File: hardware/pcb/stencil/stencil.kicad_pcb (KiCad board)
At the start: 2 copper layers, 19 x 48.2 mm, 25 parts, among them J1 USB_A, J2 Conn_01x10, J2 FH34SRJ-12S-0.5SH, J3 FH34SRJ-12S-0.5SH, J4 Conn_01x05, U2 AP2112K-3.3, U3 NC7SB3157P6X, U4 NC7SB3157P6X, U5 PRTR5V0U2X

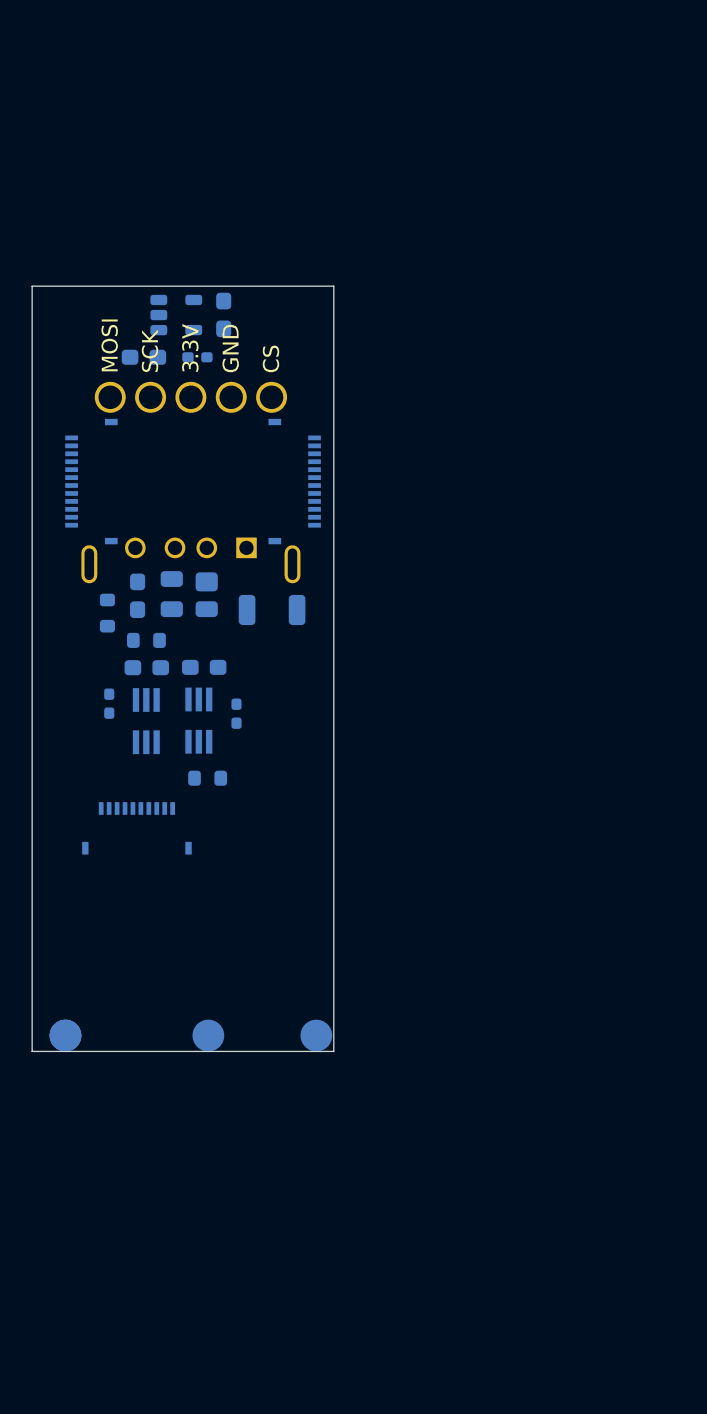
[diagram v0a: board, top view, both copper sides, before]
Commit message: production
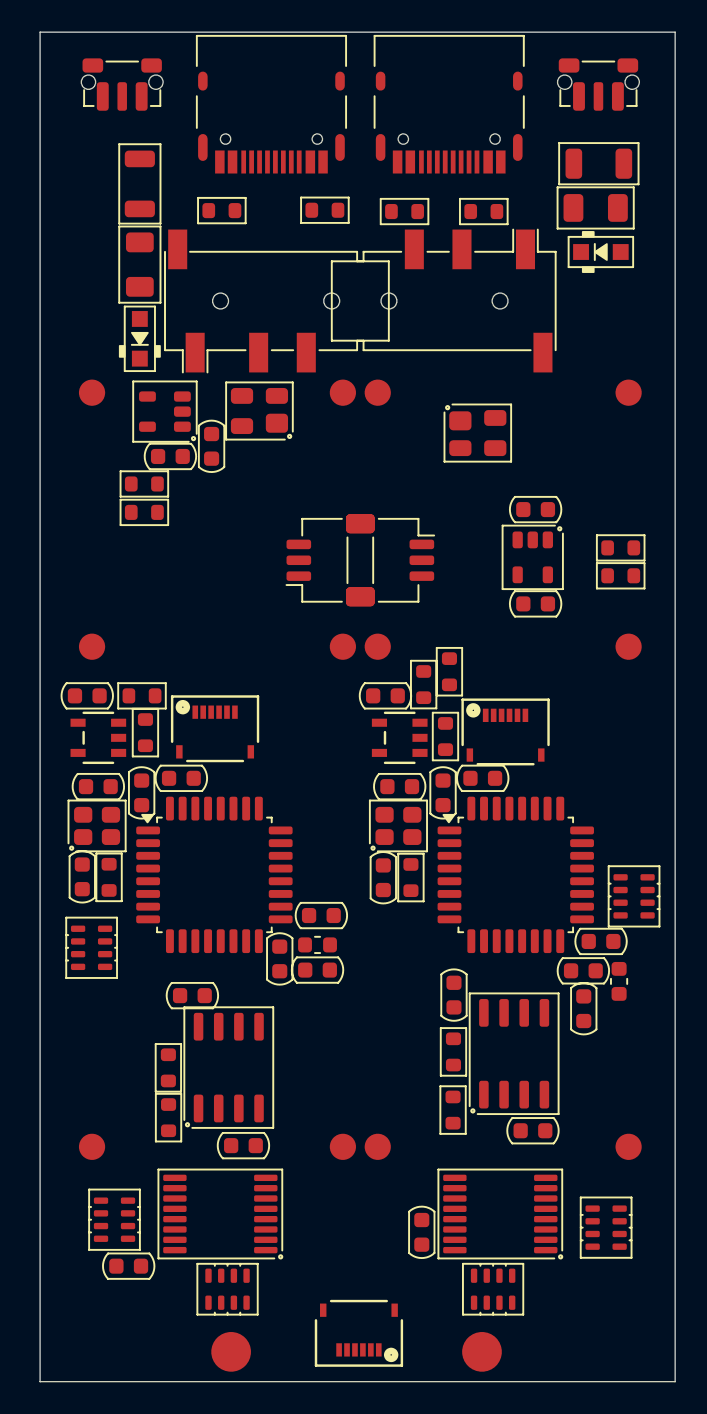
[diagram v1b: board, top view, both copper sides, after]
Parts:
- removed C1: C_Small, PCM_Capacitor_SMD_AKL:C_0603_1608Metric_Pad1.05x0.95mm
- removed the C2 at (112.1, 117.8)
- removed the C3 at (107.0, 120.5)
- removed the C6 at (110.8, 140.0)
- removed the C7 at (107.2, 140.0)
- removed the J1 at (110.0, 133.0)
- removed the J2 at (106.6, 150.1)
- removed the J2 at (103.7, 128.3)
- removed the J3 at (116.5, 128.3)
- removed the J4 at (110.0, 123.0)
- removed the L1 at (115.1, 136.4)
- removed the R1 at (110.4, 120.5)
- removed the R2 at (104.9, 142.3)
- removed the R3 at (112.9, 142.9)
- removed the R6 at (107.2, 138.3)
- removed the R7 at (111.1, 147.0)
- removed REF** (x4): NPTH, NPTH
- removed the U2 at (109.1, 117.8)
- removed the U3 at (110.5, 143.4)
- removed the U4 at (107.2, 143.4)
- removed the U5 at (109.9, 135.4)
- added C10: 220pF, PCM_Capacitor_SMD_AKL:C_0603_1608Metric, F.Cu at (131.5, 169.2)
- added C10: 220pF, PCM_Capacitor_SMD_AKL:C_0603_1608Metric, F.Cu at (113.3, 170.1)
- added C11: 4.7 uF, PCM_Capacitor_SMD_AKL:C_0603_1608Metric, F.Cu at (135.8, 157.3)
- added C12: 1u, PCM_Capacitor_SMD_AKL:C_0603_1608Metric, F.Cu at (134.7, 159.1)
- added C13: 10n, PCM_Capacitor_SMD_AKL:C_0603_1608Metric, F.Cu at (134.7, 161.5)
- added C14: 10n, PCM_Capacitor_SMD_AKL:C_0603_1608Metric, F.Cu at (103.5, 141.8)
- added C14: 10n, PCM_Capacitor_SMD_AKL:C_0603_1608Metric, F.Cu at (122.3, 141.8)
- added C15: 4.7 uF, PCM_Capacitor_SMD_AKL:C_0603_1608Metric, F.Cu at (109.4, 147.0)
- added C16: 10n, PCM_Capacitor_SMD_AKL:C_0603_1608Metric, F.Cu at (118.0, 159.1)
- added C17: 1u, PCM_Capacitor_SMD_AKL:C_0603_1608Metric, F.Cu at (115.6, 158.4)
- added C2: 0.1uF, PCM_Capacitor_SMD_AKL:C_0603_1608Metric, F.Cu at (110.1, 160.7)
- added C2: 0.1uF, PCM_Capacitor_SMD_AKL:C_0603_1608Metric, F.Cu at (126.6, 160.7)
- added C3: 0.1uF, PCM_Capacitor_SMD_AKL:C_0603_1608Metric, F.Cu at (106.1, 177.7)
- added C3: 0.1uF, PCM_Capacitor_SMD_AKL:C_0603_1608Metric, F.Cu at (124.5, 175.6)
- added C4: 0.1uF, PCM_Capacitor_SMD_AKL:C_0603_1608Metric, F.Cu at (118.2, 155.6)
- added C4: 0.1uF, PCM_Capacitor_SMD_AKL:C_0603_1608Metric, F.Cu at (128.4, 147.0)
- added C5: 0.1uF, PCM_Capacitor_SMD_AKL:C_0603_1608Metric, F.Cu at (106.9, 147.9)
- added C5: 0.1uF, PCM_Capacitor_SMD_AKL:C_0603_1608Metric, F.Cu at (125.9, 147.9)
- added C6: 10pF, PCM_Capacitor_SMD_AKL:C_0603_1608Metric, F.Cu at (104.2, 147.5)
- added C6: 10pF, PCM_Capacitor_SMD_AKL:C_0603_1608Metric, F.Cu at (123.2, 147.5)
- added C7: 10pF, PCM_Capacitor_SMD_AKL:C_0603_1608Metric, F.Cu at (103.2, 153.2)
- added C7: 10pF, PCM_Capacitor_SMD_AKL:C_0603_1608Metric, F.Cu at (122.1, 153.3)
- added C8: 1uF, PCM_Capacitor_SMD_AKL:C_0603_1608Metric, F.Cu at (108.7, 126.7)
- added C8: 1uF, PCM_Capacitor_SMD_AKL:C_0603_1608Metric, F.Cu at (131.7, 130.1)
- added C9: 1uF, PCM_Capacitor_SMD_AKL:C_0603_1608Metric, F.Cu at (111.3, 126.1)
- added C9: 1uF, PCM_Capacitor_SMD_AKL:C_0603_1608Metric, F.Cu at (131.7, 136.0)
- added D1: 1N5819, PCM_Diode_SMD_AKL:D_SOD-323_HandSoldering, F.Cu at (135.8, 113.8)
- added D1: 1N5819, PCM_Diode_SMD_AKL:D_SOD-323_HandSoldering, F.Cu at (106.8, 119.3)
- added F1: 500mA, PCM_Fuse_AKL:Fuse_1206_3216Metric, F.Cu at (106.8, 114.6)
- added F1: 500mA, PCM_Fuse_AKL:Fuse_1206_3216Metric, F.Cu at (135.5, 111.1)
- added FB1: 1kΩ 100mhz, Inductor_SMD:L_0603_1608Metric, F.Cu at (137.0, 159.8)
- added FB1: 1kΩ 100mhz, Inductor_SMD:L_0603_1608Metric, F.Cu at (118.0, 157.5)
- added H13: ~, ec_parts:SMT-SO-M1.6-screwhole_only, F.Cu at (103.8, 170.2)
- added H13: ~, ec_parts:SMT-SO-M1.6-screwhole_only, F.Cu at (137.6, 170.2)
- added H14: ~, ec_parts:SMT-SO-M1.6-screwhole_only, F.Cu at (137.6, 122.7)
- added H14: ~, ec_parts:SMT-SO-M1.6-screwhole_only, F.Cu at (103.8, 122.7)
- added H15: ~, ec_parts:SMT-SO-M1.6-screwhole_only, F.Cu at (121.8, 122.7)
- added H15: ~, ec_parts:SMT-SO-M1.6-screwhole_only, F.Cu at (119.6, 122.7)
- added H16: ~, ec_parts:SMT-SO-M1.6-screwhole_only, F.Cu at (119.6, 170.2)
- added H16: ~, ec_parts:SMT-SO-M1.6-screwhole_only, F.Cu at (121.8, 170.2)
- added H18: ~, ec_parts:SMT-SO-M1.6-screwhole_only, F.Cu at (103.8, 138.7)
- added H18: ~, ec_parts:SMT-SO-M1.6-screwhole_only, F.Cu at (121.8, 138.7)
- added H19: ~, ec_parts:SMT-SO-M1.6-screwhole_only, F.Cu at (119.6, 138.7)
- added H19: ~, ec_parts:SMT-SO-M1.6-screwhole_only, F.Cu at (137.6, 138.7)
- added H3: ~, ec_parts:SMT-SO-M1.6-with-ring, F.Cu at (128.3, 183.1)
- added H4: ~, ec_parts:SMT-SO-M1.6-with-ring, F.Cu at (112.5, 183.1)
- added J1: SM03B-SRSS-TB, Connector_JST:JST_SH_SM03B-SRSS-TB_1x03-1MP_P1.00mm_Horizontal, F.Cu at (118.8, 133.3)
- added J1: SM04B-SRSS-TB, Connector_JST:JST_SH_SM03B-SRSS-TB_1x03-1MP_P1.00mm_Horizontal, F.Cu at (122.5, 133.3)
- added J2: PJ320D, ec_parts:Jack_3.5mm_PJ320D_Horizontal, F.Cu at (114.1, 116.9)
- added J2: PJ320D, ec_parts:Jack_3.5mm_PJ320D_Horizontal, F.Cu at (127.2, 116.9)
- added J3: HRO_TYPE-C-31-M-12, ec_parts:USB_C_Receptacle_HRO_TYPE-C-31-M-12, F.Cu at (126.3, 104.1)
- added J3: HRO_TYPE-C-31-M-12, ec_parts:USB_C_Receptacle_HRO_TYPE-C-31-M-12, F.Cu at (115.1, 104.1)
- added J4: HRS_FH34SRJ-06S-0.5SH(50), ec_parts:CONN6x1_FH34SRJ-6S-0.5SH50_HIR, F.Cu at (129.8, 144.1)
- added J4: HRS_FH34SRJ-06S-0.5SH(50), ec_parts:CONN6x1_FH34SRJ-6S-0.5SH50_HIR, F.Cu at (120.6, 182.0)
- added J4: HRS_FH34SRJ-06S-0.5SH(50), ec_parts:CONN6x1_FH34SRJ-6S-0.5SH50_HIR, F.Cu at (111.5, 143.9)
- added L1: 60R@100MHz, PCM_Inductor_SMD_AKL:L_1206_3216Metric, F.Cu at (106.8, 109.6)
- added L1: 60R@100MHz, PCM_Inductor_SMD_AKL:L_1206_3216Metric, F.Cu at (135.7, 108.3)
- added R1: 10k, PCM_Resistor_SMD_AKL:R_0603_1608Metric, F.Cu at (123.9, 153.2)
- added R1: 10k, PCM_Resistor_SMD_AKL:R_0603_1608Metric, F.Cu at (107.1, 128.5)
- added R10: 10k, PCM_Resistor_SMD_AKL:R_0603_1608Metric, F.Cu at (126.0, 144.4)
- added R10: 10k, PCM_Resistor_SMD_AKL:R_0603_1608Metric, F.Cu at (107.1, 144.1)
- added R2: 5.1k, PCM_Resistor_SMD_AKL:R_0603_1608Metric, F.Cu at (118.4, 111.2)
- added R2: 5.1k, PCM_Resistor_SMD_AKL:R_0603_1608Metric, F.Cu at (128.4, 111.3)
- added R3: 5.1k, PCM_Resistor_SMD_AKL:R_0603_1608Metric, F.Cu at (123.5, 111.3)
- added R3: 5.1k, PCM_Resistor_SMD_AKL:R_0603_1608Metric, F.Cu at (111.9, 111.2)
- added R4: 10k, PCM_Resistor_SMD_AKL:R_0603_1608Metric, F.Cu at (137.1, 132.5)
- added R4: 5.1k, PCM_Resistor_SMD_AKL:R_0603_1608Metric, F.Cu at (107.1, 130.2)
- added R6: 1k, PCM_Resistor_SMD_AKL:R_0603_1608Metric, F.Cu at (126.5, 167.9)
- added R6: 1k, PCM_Resistor_SMD_AKL:R_0603_1608Metric, F.Cu at (108.6, 168.4)
- added R7: 100k, PCM_Resistor_SMD_AKL:R_0603_1608Metric, F.Cu at (126.5, 164.2)
- added R7: 100k, PCM_Resistor_SMD_AKL:R_0603_1608Metric, F.Cu at (108.6, 165.2)
- added R8: 10k, PCM_Resistor_SMD_AKL:R_0603_1608Metric, F.Cu at (104.8, 153.2)
- added R8: 1k, PCM_Resistor_SMD_AKL:R_0603_1608Metric, F.Cu at (126.3, 140.3)
- added R9: 10k, PCM_Resistor_SMD_AKL:R_0603_1608Metric, F.Cu at (124.7, 141.1)
- added R9: 10k, PCM_Resistor_SMD_AKL:R_0603_1608Metric, F.Cu at (106.9, 141.8)
- added RN1: 100k R_Array_Concave_4x0603, PCM_Resistor_SMD_AKL:R_Array_Concave_4x0603, F.Cu at (136.2, 175.3)
- added RN1: 100k R_Array_Concave_4x0603, PCM_Resistor_SMD_AKL:R_Array_Concave_4x0603, F.Cu at (105.2, 174.8)
- added RN2: 100k R_Array_Concave_4x0603, PCM_Resistor_SMD_AKL:R_Array_Concave_4x0603, F.Cu at (129.0, 179.2)
- added RN2: 100k R_Array_Concave_4x0603, PCM_Resistor_SMD_AKL:R_Array_Concave_4x0603, F.Cu at (112.3, 179.2)
- added RN3: 100 R_Array_Convex_4x0603, PCM_Resistor_SMD_AKL:R_Array_Concave_4x0603, F.Cu at (137.9, 154.4)
- added RN3: 100 R_Array_Convex_4x1206, PCM_Resistor_SMD_AKL:R_Array_Concave_4x0603, F.Cu at (103.7, 157.7)
- added SW29: PTS845, Button_Switch_SMD:SW_Push_1P1T-MP_NO_Horizontal_Alps_SKRTLAE010, F.Cu at (105.7, 103.2)
- added SW29: PTS845, Button_Switch_SMD:SW_Push_1P1T-MP_NO_Horizontal_Alps_SKRTLAE010, F.Cu at (135.7, 103.2)
- added U1: 74HC4051, PCM_Package_SO_AKL:TSSOP-16_4.4x5mm_P0.65mm, F.Cu at (111.9, 174.4)
- added U1: 74HC4051, PCM_Package_SO_AKL:TSSOP-16_4.4x5mm_P0.65mm, F.Cu at (129.5, 174.4)
- added U2: OPA350UA, PCM_Package_SO_AKL:SO-8_3.9x4.9mm_P1.27mm, F.Cu at (112.4, 165.2)
- added U2: OPA350UA, PCM_Package_SO_AKL:SO-8_3.9x4.9mm_P1.27mm, F.Cu at (130.4, 164.3)
- added U3: PRTR5V0U2X, PCM_Package_TO_SOT_SMD_AKL:SOT-143, F.Cu at (114.3, 123.9)
- added U3: PRTR5V0U2X, PCM_Package_TO_SOT_SMD_AKL:SOT-143, F.Cu at (128.1, 125.3)
- added U4: XC6220B331MR-G, PCM_Package_TO_SOT_SMD_AKL:SOT-23-5, F.Cu at (131.5, 133.1)
- added U4: XC6220B331MR-G, PCM_Package_TO_SOT_SMD_AKL:SOT-23-5, F.Cu at (108.4, 123.9)
- added U5: STM32G431KBTx, Package_QFP:LQFP-32_7x7mm_P0.8mm, F.Cu at (111.5, 153.1)
- added U5: STM32G431KBTx, Package_QFP:LQFP-32_7x7mm_P0.8mm, F.Cu at (130.5, 153.1)
- added U6: 24FC01T-I/OT, ec_parts:SOT-23-5_2P9X1P6_MCH, F.Cu at (104.2, 144.4)
- added U6: 24FC01T-I/OT, ec_parts:SOT-23-5_2P9X1P6_MCH, F.Cu at (123.2, 144.4)
- added Y1: 8MHz 10pF, PCM_Crystal_Handsoldering_AKL:Crystal_SMD_2520-4Pin_2.5x2.0mm, F.Cu at (104.1, 150.0)
- added Y1: 8MHz 10pF, PCM_Crystal_Handsoldering_AKL:Crystal_SMD_2520-4Pin_2.5x2.0mm, F.Cu at (123.1, 150.0)
- R5: value 10k -> 5.1k; moved to F.Cu
- moved R5 32.4 mm to (137.1, 134.2), turned to 180 degrees
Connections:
- R5 pad 1: (no net) -> GND
- R5 pad 2: (no net) -> PB6
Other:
- board size 19 x 48.2 mm -> 40 x 85 mm
